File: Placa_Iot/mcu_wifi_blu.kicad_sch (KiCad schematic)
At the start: 0 parts

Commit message: mricro con conector
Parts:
- added C10, C11, C5: 10 nF, Capacitor_SMD:C_0402_1005Metric, symbol Device:C
- added C12, C13: 12 pF, Capacitor_SMD:C_0402_1005Metric, symbol Device:C
- added C14, C15, C16, C17, C18, C19: NC, Capacitor_SMD:C_0402_1005Metric, symbol Device:C
- added C20, C21, C7: 100 nF, Capacitor_SMD:C_0402_1005Metric, symbol Device:C
- added C6, C8, C9: 1 uF, Capacitor_SMD:C_0402_1005Metric, symbol Device:C
- added J1, J2: 22-28-4144, connectors:CONN_THT_MV_PH_P2.54MM_P14, symbol connectors:CONN_THT_MV_PH_P2.54MM_P14
- added L1: 2 nH, Resistor_SMD:R_0402_1005Metric, symbol Device:L
- added L2: 22 nH, Resistor_SMD:R_0402_1005Metric, symbol Device:L
- added R4, R5: NC, Resistor_SMD:R_0402_1005Metric, symbol resistor:R
- added R6, R7: 10 kOhm, Resistor_SMD:R_0402_1005Metric, symbol resistor:R
- added SW1, SW2: SW_Push, Button_Switch_SMD:SW_Push_SPST_NO_Alps_SKRK, symbol Switch:SW_Push
- added U3: ESP32-S3, ic_control:QFN-56-1EP_7x7mm_P0.4mm_EP4x4mm, symbol ic_control:ESP32-S3
- added U4: PRO-OB-536, antennas:ANTENNA_PIFA_3D_2.4GHZ, symbol antenas:ANTENNA_PIFA_3D_2.4GHZ
- added Y1: 40 Mhz, Crystal:Crystal_SMD_3225-4Pin_3.2x2.5mm, symbol Device:Crystal_GND24
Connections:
- new net: C14.2, C15.1, C17.1, C18.1
- new net: C18.2, C19.1, U4.2 (FEED)
- new net: C14.1, C16.1, U3.1 (LNA_IN)
- new net: C11.1, L1.2, U3.2 (VDD3P3), U3.3 (VDD3P3)
- new net: R5.2, U3.49 (U0TXD)
- new net: C13.1, U3.53 (XTAL_N), Y1.3
- new net: L2.2, U3.54 (XTAL_P)
- new net: C12.1, L2.1, Y1.1
- new net +3.3V: C10.1, C20.1, C5.1, C6.1, C7.1, C8.1, C9.1, L1.1, R4.2, R6.2, R7.2, U3.20 (VDD3P3_RTC), U3.46 (VDD3P3_CPU), U3.55 (VDDA), U3.56 (VDDA)
- new net 100: R7.1, SW2.1
- new net CLK-SCK-IO14: U3.19 (GPIO14)
- new net CMD-MOSI-IO11: U3.16 (GPIO11)
- new net DM: U3.25 (GPIO19/USB_D-)
- new net DP: U3.26 (GPIO20/USB_D+)
- new net GND: C10.2, C11.2, C12.2, C13.2, C16.2, C17.2, C19.2, C20.2, C21.2, C5.2, C6.2, C7.2, C8.2, C9.2, J1.2 (Pin_2), J1.4 (Pin_4), SW1.2, SW2.2, U3.57 (GND), U4.1 (GND), Y1.2 (G), Y1.4 (G)
- new net IO0: J2.3 (Pin_3), U3.5 (GPIO0)
- new net IO1: U3.6 (GPIO1)
- new net IO12: J2.10 (Pin_10), U3.17 (GPIO12)
- new net IO15: J2.12 (Pin_12), U3.21 (XTAL_32K_P)
- new net IO16: J2.13 (Pin_13), U3.22 (XTAL_32K_N)
- new net IO17: U3.23 (GPIO17)
- new net IO18: U3.24 (GPIO18)
- new net IO3: U3.8 (GPIO3)
- new net IO33: J2.14 (Pin_14), J2.6 (Pin_6), U3.38 (GPIO33)
- new net IO34: J2.5 (Pin_5), U3.39 (GPIO34)
- new net IO35: J2.4 (Pin_4), U3.40 (GPIO35)
- new net IO36: J2.2 (Pin_2), U3.41 (GPIO36)
- new net IO37: J2.1 (Pin_1), U3.42 (GPIO37)
- new net IO38: J1.13 (Pin_13), U3.43 (GPIO38)
- new net IO39/MTCK: J1.10 (Pin_10)
- new net IO39/MTCX: U3.44 (MTCK)
- new net IO4: U3.9 (GPIO4)
- new net IO40/MTDO: J1.9 (Pin_9), U3.45 (MTDO)
- new net IO41/MTD1: U3.47 (MTDI)
- new net IO41/MTDI: J1.8 (Pin_8)
- new net IO42/MTMS: J1.5 (Pin_5), U3.48 (MTMS)
- new net IO45: J1.7 (Pin_7), R4.1, U3.51 (GPIO45)
- new net IO46: J1.6 (Pin_6), U3.52 (GPIO46)
- new net IO47: J2.7 (Pin_7), U3.37 (SPICLK_P)
- new net IO48: J2.8 (Pin_8), U3.36 (SPICLK_N)
- new net IO5: U3.10 (GPIO5)
- new net IO6: U3.11 (GPIO6)
- new net IO7: U3.12 (GPIO7)
- new net IO8: J2.9 (Pin_9), U3.13 (GPIO8)
- new net IO9: U3.14 (GPIO9)
- new net LORA_RDX: U3.27 (GPIO21)
- new net LORA_TX: U3.15 (GPIO10)
- new net RST/EN: J2.11 (Pin_11)
- new net RST/EN: C21.1, R6.1, SW1.1, U3.4 (CHIP_PU)
- new net SD0-MISO-IO2: U3.7 (GPIO2)
- new net SD3-CS-IO13: U3.18 (GPIO13)
- new net UORXD: J1.11 (Pin_11), U3.50 (U0RXD)
- new net UOTXD: J1.12 (Pin_12), R5.1
- new net VBAT: J1.14 (Pin_14)
- new net VBUS: J1.1 (Pin_1)
- new net VCC3V3: J1.3 (Pin_3)
- no-connect marks 0 -> 8

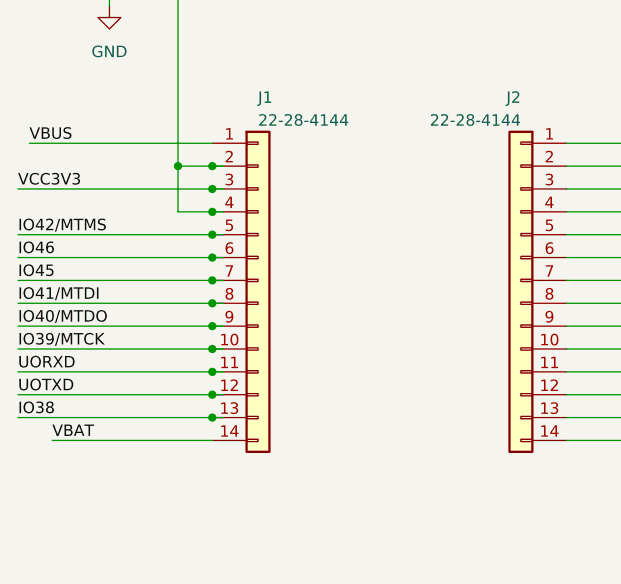
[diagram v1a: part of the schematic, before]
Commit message: RF commit
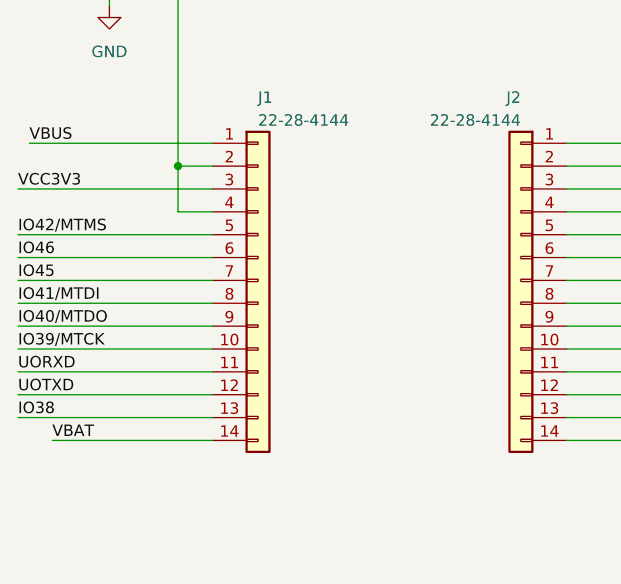
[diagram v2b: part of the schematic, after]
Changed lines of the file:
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@@
 	(paper "A3")
 	(junction
-		(at 35.56 143.51)
-		(diameter 0)
-		(color 0 0 0 0)
-	)
-	(junction
-		(at 35.56 153.67)
-		(diameter 0)
-		(color 0 0 0 0)
-	)
-	(junction
 		(at 116.84 210.82)
 		(diameter 0)
@@
 	)
 	(junction
-		(at 35.56 156.21)
-		(diameter 0)
-		(color 0 0 0 0)
-	)
-	(junction
 		(at 200.66 102.87)
 		(diameter 0)
@@
 	)
 	(junction
-		(at 35.56 163.83)
-		(diameter 0)
-		(color 0 0 0 0)
-	)
-	(junction
-		(at 35.56 158.75)
-		(diameter 0)
-		(color 0 0 0 0)
-	)
-	(junction
-		(at 35.56 151.13)
-		(diameter 0)
-		(color 0 0 0 0)
-	)
-	(junction
 		(at 184.15 66.04)
 		(diameter 0)
@@
 	)
 	(junction
-		(at 35.56 146.05)
-		(diameter 0)
-		(color 0 0 0 0)
-	)
-	(junction
 		(at 166.37 124.46)
 		(diameter 0)
@@
 	)
 	(junction
-		(at 35.56 148.59)
-		(diameter 0)
-		(color 0 0 0 0)
-	)
-	(junction
 		(at 148.59 144.78)
 		(diameter 0)
@@
 	(junction
 		(at 275.59 193.04)
-		(diameter 0)
-		(color 0 0 0 0)
-	)
-	(junction
-		(at 35.56 140.97)
-		(diameter 0)
-		(color 0 0 0 0)
-	)
-	(junction
-		(at 35.56 138.43)
-		(diameter 0)
-		(color 0 0 0 0)
-	)
-	(junction
-		(at 35.56 161.29)
-		(diameter 0)
-		(color 0 0 0 0)
-	)
-	(junction
-		(at 35.56 135.89)
 		(diameter 0)
 		(color 0 0 0 0)
@@
 	(wire
 		(pts
-			(xy 35.56 161.29) (xy 36.83 161.29)
-		)
-		(stroke
-			(width 0)
-			(type default)
-		)
-	)
-	(wire
-		(pts
 			(xy 31.75 140.97) (xy 35.56 140.97)
 		)
@@
 	(wire
 		(pts
-			(xy 35.56 158.75) (xy 36.83 158.75)
-		)
-		(stroke
-			(width 0)
-			(type default)
-		)
-	)
-	(wire
-		(pts
 			(xy 217.17 160.02) (xy 194.31 160.02)
 		)
@@
 	(wire
 		(pts
-			(xy 35.56 135.89) (xy 36.83 135.89)
-		)
-		(stroke
-			(width 0)
-			(type default)
-		)
-	)
-	(wire
-		(pts
 			(xy 13.97 163.83) (xy 35.56 163.83)
 		)
@@
 	(wire
 		(pts
-			(xy 35.56 151.13) (xy 36.83 151.13)
-		)
-		(stroke
-			(width 0)
-			(type default)
-		)
-	)
-	(wire
-		(pts
 			(xy 24.13 111.76) (xy 24.13 118.11)
 		)
@@
 	(wire
 		(pts
-			(xy 35.56 146.05) (xy 36.83 146.05)
-		)
-		(stroke
-			(width 0)
-			(type default)
-		)
-	)
-	(wire
-		(pts
 			(xy 161.29 102.87) (xy 163.83 102.87)
 		)
@@
 	(wire
 		(pts
-			(xy 35.56 138.43) (xy 36.83 138.43)
-		)
-		(stroke
-			(width 0)
-			(type default)
-		)
-	)
-	(wire
-		(pts
-			(xy 35.56 153.67) (xy 36.83 153.67)
-		)
-		(stroke
-			(width 0)
-			(type default)
-		)
-	)
-	(wire
-		(pts
 			(xy 232.41 207.01) (xy 232.41 208.28)
 		)
@@
 	(wire
 		(pts
-			(xy 35.56 148.59) (xy 36.83 148.59)
-		)
-		(stroke
-			(width 0)
-			(type default)
-		)
-	)
-	(wire
-		(pts
-			(xy 35.56 140.97) (xy 36.83 140.97)
-		)
-		(stroke
-			(width 0)
-			(type default)
-		)
-	)
-	(wire
-		(pts
 			(xy 217.17 162.56) (xy 194.31 162.56)
 		)
@@
 	(wire
 		(pts
-			(xy 35.56 156.21) (xy 36.83 156.21)
-		)
-		(stroke
-			(width 0)
-			(type default)
-		)
-	)
-	(wire
-		(pts
 			(xy 96.52 135.89) (xy 74.93 135.89)
 		)
@@
 	(wire
 		(pts
-			(xy 35.56 163.83) (xy 36.83 163.83)
-		)
-		(stroke
-			(width 0)
-			(type default)
-		)
-	)
-	(wire
-		(pts
 			(xy 127 102.87) (xy 109.22 102.87)
 		)
@@
 		)
 		(stroke
-			(width 0)
-			(type default)
-		)
-	)
-	(wire
-		(pts
-			(xy 35.56 143.51) (xy 36.83 143.51)
-		)
-		(stroke
